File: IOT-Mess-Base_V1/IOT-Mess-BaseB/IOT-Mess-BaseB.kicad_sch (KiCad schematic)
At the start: 23 parts, among them J1 Milk-V Duo, J2 SuperMini_ESP32-H2, J4 Lolin32-Lite, J8 Luat32 C3, SW3 SW_Push, U1 SHT4x, U12 APDS-9960, U13 SHT31-DIS, U17 BH1750FVI-TR, U3 INA219AxDCN

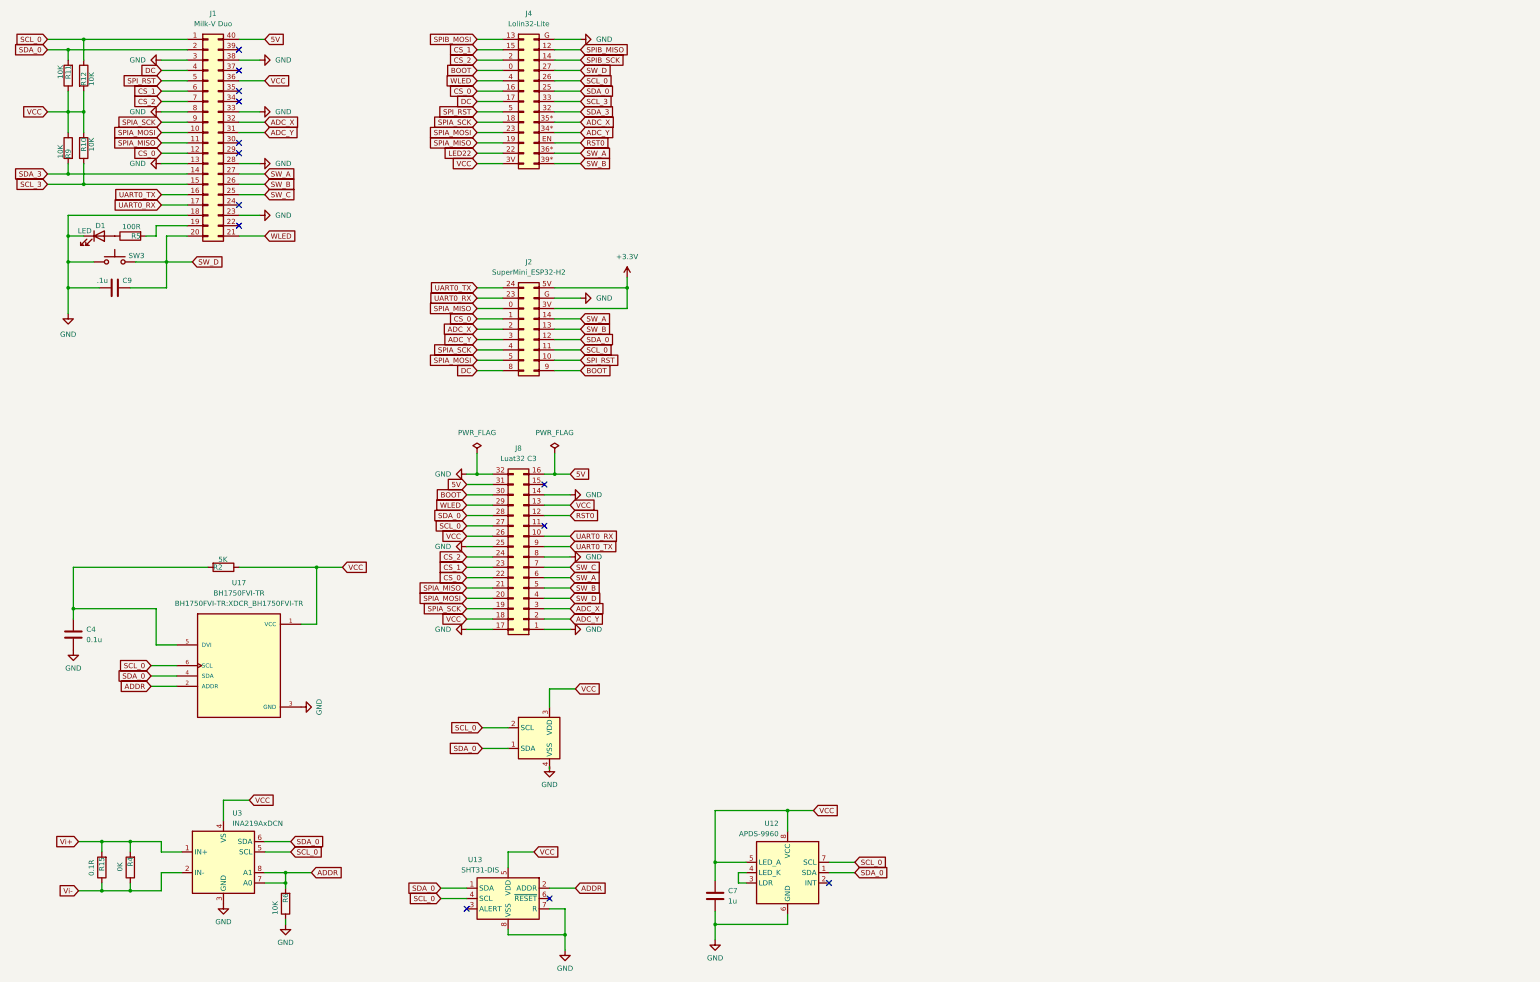
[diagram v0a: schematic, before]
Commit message: did some works.
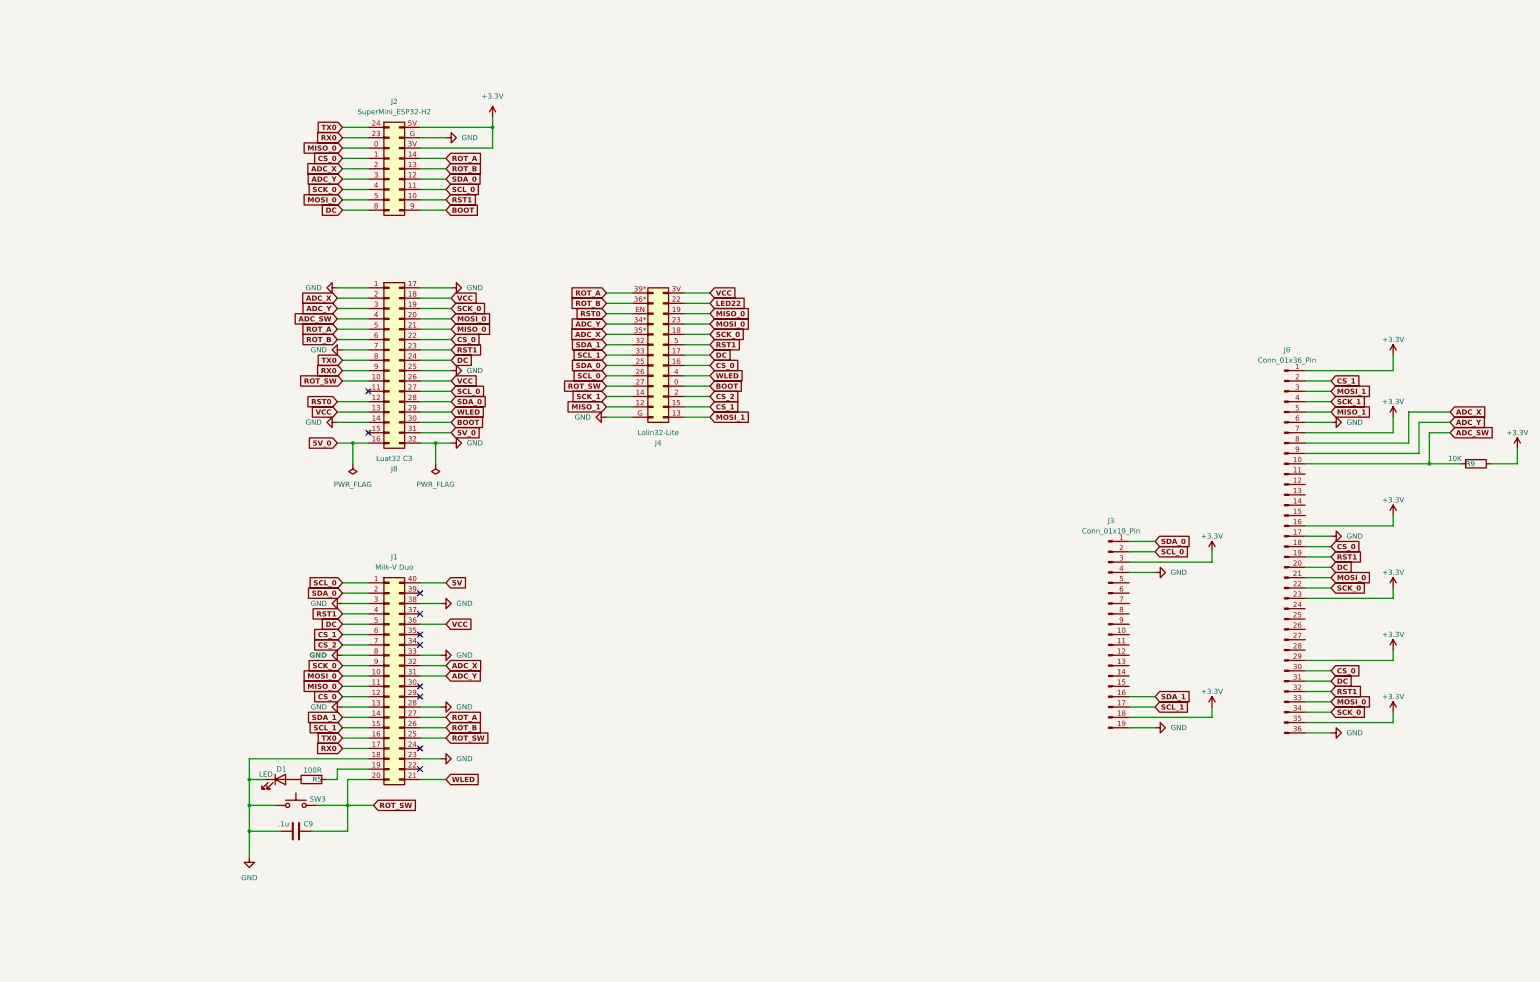
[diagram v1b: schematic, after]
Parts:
- removed C4: 0.1u, Capacitor_SMD:C_0603_1608Metric, symbol Device:C
- removed C7: 1u, Capacitor_SMD:C_0603_1608Metric, symbol Device:C
- removed R10, R11, R12, R6: 10K, Resistor_SMD:R_0603_1608Metric, symbol Device:R
- removed R15: 0.1R, Resistor_SMD:R_2512_6332Metric, symbol Device:R
- removed R2: 5K, Resistor_SMD:R_0603_1608Metric, symbol Device:R
- removed R4: 0K, Jumper:SolderJumper-2_P1.3mm_Open_Pad1.0x1.5mm, symbol Device:R
- removed U1: SHT4x, Sensor_Humidity:Sensirion_DFN-4_1.5x1.5mm_P0.8mm_SHT4x_NoCentralPad, symbol Sensor_Humidity:SHT4x
- removed U12: APDS-9960, Sensor:Avago_APDS-9960, symbol Sensor:APDS-9960
- removed U13: SHT31-DIS, Sensor_Humidity:Sensirion_DFN-8-1EP_2.5x2.5mm_P0.5mm_EP1.1x1.7mm, symbol Sensor_Humidity:SHT31-DIS
- removed U17: BH1750FVI-TR, BH1750FVI-TR:XDCR_BH1750FVI-TR, symbol BH1750FVI-TR:BH1750FVI-TR
- removed U3: INA219AxDCN, Package_TO_SOT_SMD:SOT-23-8, symbol Sensor_Energy:INA219AxDCN
- added J3: Conn_01x19_Pin, Connector_PinHeader_2.54mm:PinHeader_1x19_P2.54mm_Vertical, symbol Connector:Conn_01x19_Pin
- added J6: Conn_01x36_Pin, Connector_PinHeader_2.54mm:PinHeader_1x36_P2.54mm_Vertical, symbol Connector:Conn_01x36_Pin
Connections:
- net +3.3V: now also R9.1, J3.18 (Pin_18), J3.3 (Pin_3), J6.1 (Pin_1), J6.16 (Pin_16), J6.23 (Pin_23), J6.29 (Pin_29), J6.35 (Pin_35), J6.7 (Pin_7)
- net 5V: no longer J8.16 (Pin_16), J8.31 (Pin_31)
- net ADC_X: now also J8.2 (Pin_2), J6.8 (Pin_8); no longer J8.3 (Pin_3)
- net ADC_Y: now also J8.3 (Pin_3), J6.9 (Pin_9); no longer J8.2 (Pin_2)
- net CS_0: now also J6.18 (Pin_18), J6.30 (Pin_30)
- net CS_1: now also J6.2 (Pin_2); no longer J8.23 (Pin_23)
- net CS_2: no longer J8.24 (Pin_24)
- net DC: now also J1.5 (Pin_5), J8.24 (Pin_24), J6.20 (Pin_20), J6.31 (Pin_31); no longer J1.4 (Pin_4)
- net GND: now also J8.7 (Pin_7), J3.19 (Pin_19), J3.4 (Pin_4), J6.17 (Pin_17), J6.36 (Pin_36), J6.6 (Pin_6); no longer J8.8 (Pin_8)
- net SCL_0: now also J3.2 (Pin_2)
- net SDA_0: now also J3.1 (Pin_1)
- net VCC: no longer R9.1
- net SCL_3 renamed SCL_1
- net SCL_1: now also J3.17 (Pin_17)
- net SDA_3 renamed SDA_1
- net SDA_1: now also J3.16 (Pin_16); no longer R9.2
- net SPIA_MISO renamed MISO_0
- net SPIA_MOSI renamed MOSI_0
- net MOSI_0: now also J6.21 (Pin_21), J6.33 (Pin_33)
- net SPIA_SCK renamed SCK_0
- net SCK_0: now also J6.22 (Pin_22), J6.34 (Pin_34)
- net SPIB_MISO renamed MISO_1
- net MISO_1: now also J6.5 (Pin_5)
- net SPIB_MOSI renamed MOSI_1
- net MOSI_1: now also J6.3 (Pin_3)
- net SPIB_SCK renamed SCK_1
- net SCK_1: now also J6.4 (Pin_4)
- net SPI_RST renamed RST1
- net RST1: now also J1.4 (Pin_4), J8.23 (Pin_23), J6.19 (Pin_19), J6.32 (Pin_32); no longer J1.5 (Pin_5)
- net SW_A renamed ROT_A
- net ROT_A: now also J4.39* (Pin_13b), J8.5 (Pin_5); no longer J4.36* (Pin_12b), J8.6 (Pin_6)
- net SW_B renamed ROT_B
- net ROT_B: now also J4.36* (Pin_12b), J8.6 (Pin_6); no longer J4.39* (Pin_13b), J8.5 (Pin_5)
- net SW_C renamed ROT_SW
- net ROT_SW: now also C9.2, J1.20 (Pin_20), J4.27 (Pin_4b), J8.10 (Pin_10), SW3.1; no longer J8.7 (Pin_7)
- removed net SW_D: C9.2, J1.20 (Pin_20), J4.27 (Pin_4b), J8.4 (Pin_4), SW3.1
- net UART0_RX renamed RX0
- net RX0: now also J8.9 (Pin_9); no longer J8.10 (Pin_10)
- net UART0_TX renamed TX0
- net TX0: now also J8.8 (Pin_8); no longer J8.9 (Pin_9)
- new net 5V_0: J8.16 (Pin_16), J8.31 (Pin_31)
- new net ADC_SW: J6.10 (Pin_10), J8.4 (Pin_4), R9.2
- no-connect marks 13 -> 10
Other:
- moved on the sheet: C9, D1, J1, J2, J4, J8, R5, SW3

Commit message: did some works.
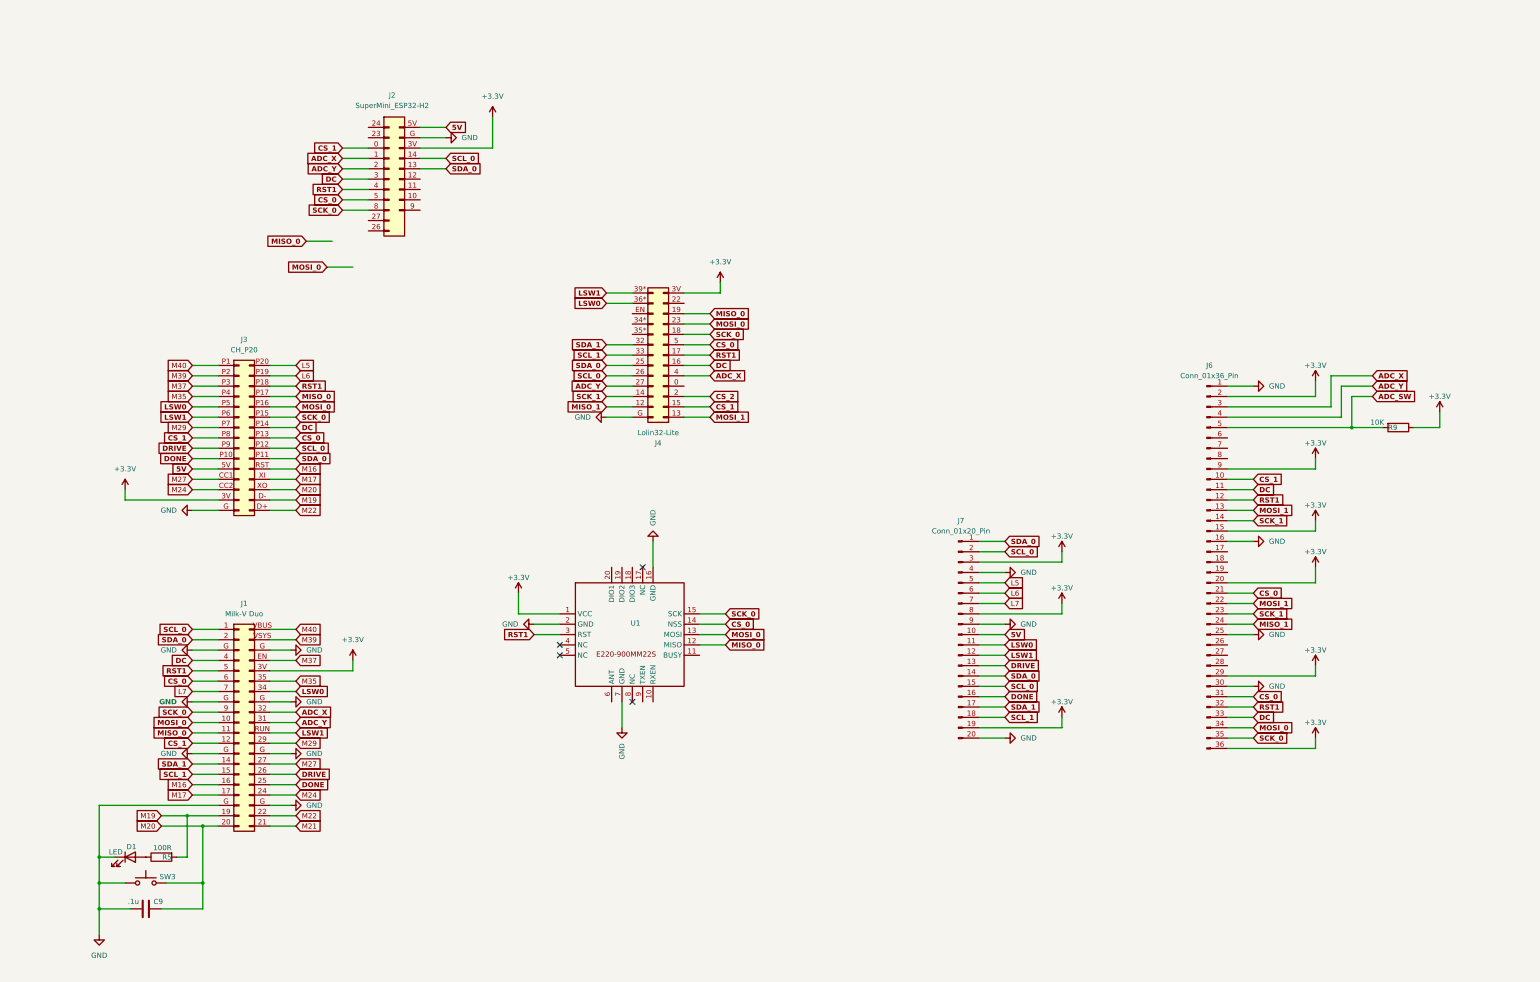
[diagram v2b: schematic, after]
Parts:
- removed J3: Conn_01x19_Pin, Connector_PinHeader_2.54mm:PinHeader_1x19_P2.54mm_Vertical, symbol Connector:Conn_01x19_Pin
- removed J8: Luat32 C3, IOT-Mess-Footprints:Luat32 C3, symbol Connector_Generic:Conn_02x16_Top_Bottom
- added J3: CH_P20, IOT-Mess-Footprints:CH_P20, symbol IOT-Mess:CH_P20
- added J7: Conn_01x20_Pin, Connector_PinHeader_2.54mm:PinHeader_1x20_P2.54mm_Vertical, symbol Connector:Conn_01x20_Pin
- added U1: ~, IOT-Mess-Footprints:E220-900, symbol IOT-Mess:E220-900
- J2: footprint (none) -> IOT-Mess-Footprints:SuperMiniH2
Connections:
- net +3.3V: now also J1.3V (Pin_36), J4.3V (Pin_13a), J6.15 (Pin_15), J6.2 (Pin_2), J6.20 (Pin_20), J6.36 (Pin_36), J6.9 (Pin_9), J3.3V (Pin_14), J7.19 (Pin_19), J7.3 (Pin_3), J7.8 (Pin_8), U1.1 (VCC); no longer J2.5V (Pin_18), J6.1 (Pin_1), J6.16 (Pin_16), J6.23 (Pin_23), J6.35 (Pin_35), J6.7 (Pin_7)
- net 5V: now also J2.5V (Pin_18), J3.5V (Pin_11), J7.10 (Pin_10); no longer J1.40 (Pin_40)
- net ADC_SW: now also J6.5 (Pin_5); no longer J6.10 (Pin_10)
- net ADC_X: now also J2.1 (Pin_4), J4.4 (Pin_5a), J6.3 (Pin_3); no longer J2.2 (Pin_5), J4.35* (Pin_9b), J6.8 (Pin_8)
- net ADC_Y: now also J2.2 (Pin_5), J4.27 (Pin_4b), J6.4 (Pin_4); no longer J2.3 (Pin_6), J4.34* (Pin_10b), J6.9 (Pin_9)
- net CS_0: now also J1.6 (Pin_6), J2.5 (Pin_8), J4.5 (Pin_8a), J6.21 (Pin_21), J6.31 (Pin_31), J3.P13 (Pin_23), U1.14 (NSS); no longer J1.12 (Pin_12), J2.1 (Pin_4), J4.16 (Pin_6a), J6.18 (Pin_18), J6.30 (Pin_30)
- net CS_1: now also J1.12 (Pin_12), J2.0 (Pin_3), J6.10 (Pin_10), J3.P8 (Pin_8); no longer J1.6 (Pin_6), J6.2 (Pin_2)
- net CS_2: no longer J1.7 (Pin_7)
- net DC: now also J1.4 (Pin_4), J2.3 (Pin_6), J4.16 (Pin_6a), J6.11 (Pin_11), J6.33 (Pin_33), J3.P14 (Pin_22); no longer J1.5 (Pin_5), J2.8 (Pin_9), J4.17 (Pin_7a), J6.20 (Pin_20), J6.31 (Pin_31)
- net GND: now also J1.G (Pin_23), J6.1 (Pin_1), J6.16 (Pin_16), J6.25 (Pin_25), J6.30 (Pin_30), J3.G (Pin_15), J7.20 (Pin_20), J7.4 (Pin_4), J7.9 (Pin_9), U1.16 (GND), U1.2 (GND), U1.7 (GND); no longer J1.13 (Pin_13), J1.18 (Pin_18), J1.23 (Pin_23), J1.28 (Pin_28), J1.3 (Pin_3), J1.33 (Pin_33), J1.38 (Pin_38), J1.8 (Pin_8), J6.17 (Pin_17), J6.36 (Pin_36), J6.6 (Pin_6)
- net MISO_0: now also J3.P17 (Pin_19), U1.12 (MISO); no longer J2.0 (Pin_3)
- net MISO_1: now also J6.24 (Pin_24); no longer J6.5 (Pin_5)
- net MOSI_0: now also J6.34 (Pin_34), J3.P16 (Pin_20), U1.13 (MOSI); no longer J2.5 (Pin_8), J6.21 (Pin_21), J6.33 (Pin_33)
- net MOSI_1: now also J6.13 (Pin_13), J6.22 (Pin_22); no longer J6.3 (Pin_3)
- net RST1: now also J1.5 (Pin_5), J2.4 (Pin_7), J4.17 (Pin_7a), J6.12 (Pin_12), J3.P18 (Pin_18), U1.3 (RST); no longer J1.4 (Pin_4), J2.10 (Pin_11), J4.5 (Pin_8a), J6.19 (Pin_19)
- net SCK_0: now also J2.8 (Pin_9), J6.35 (Pin_35), J3.P15 (Pin_21), U1.15 (SCK); no longer J2.4 (Pin_7), J6.22 (Pin_22), J6.34 (Pin_34)
- net SCK_1: now also J6.14 (Pin_14), J6.23 (Pin_23); no longer J6.4 (Pin_4)
- net SCL_0: now also J2.14 (Pin_15), J3.P12 (Pin_24), J7.15 (Pin_15), J7.2 (Pin_2); no longer J2.11 (Pin_12)
- net SCL_1: now also J7.18 (Pin_18)
- net SDA_0: now also J2.13 (Pin_14), J3.P11 (Pin_25), J7.1 (Pin_1), J7.14 (Pin_14); no longer J2.12 (Pin_13)
- net SDA_1: now also J7.17 (Pin_17)
- net M19: now reaches J1.19 (Pin_19), R5.2
- net M19: now also J3.D- (Pin_29)
- net M22: now reaches J1.22 (Pin_22)
- net M22: now also J3.D+ (Pin_30)
- net M24: now reaches J1.24 (Pin_24)
- net M24: now also J3.CC2 (Pin_13)
- net M29: now reaches J1.29 (Pin_29)
- net M29: now also J3.P7 (Pin_7)
- net LSW0: now reaches J1.34 (Pin_34)
- net LSW0: now also J4.36* (Pin_12b), J3.P5 (Pin_5), J7.11 (Pin_11)
- net M35: now reaches J1.35 (Pin_35)
- net M35: now also J3.P4 (Pin_4)
- net BOOT: no longer names the net of J4.0 (Pin_4a)
- net BOOT: no longer J2.9 (Pin_10)
- net LED22: no longer names the net of J4.22 (Pin_12a)
- removed net ROT_A: J1.27 (Pin_27), J2.14 (Pin_15), J4.39* (Pin_13b)
- removed net ROT_B: J1.26 (Pin_26), J2.13 (Pin_14), J4.36* (Pin_12b)
- net ROT_SW renamed M20
- net M20: now also J3.XO (Pin_28); no longer J1.25 (Pin_25), J4.27 (Pin_4b)
- net RST0: no longer names the net of J4.EN (Pin_11b)
- net RX0: no longer names the net of J2.23 (Pin_2)
- net RX0: no longer J1.17 (Pin_17)
- net TX0: no longer names the net of J2.24 (Pin_1)
- net TX0: no longer J1.16 (Pin_16)
- removed net VCC: J1.36 (Pin_36), J4.3V (Pin_13a)
- net WLED renamed M21
- net M21: no longer J4.4 (Pin_5a)
- new net DONE: J1.25 (Pin_25), J3.P10 (Pin_10), J7.16 (Pin_16)
- new net DRIVE: J1.26 (Pin_26), J3.P9 (Pin_9), J7.13 (Pin_13)
- new net L5: J3.P20 (Pin_16), J7.5 (Pin_5)
- new net L6: J3.P19 (Pin_17), J7.6 (Pin_6)
- new net L7: J1.7 (Pin_7), J7.7 (Pin_7)
- new net LSW1: J1.RUN (Pin_30), J3.P6 (Pin_6), J4.39* (Pin_13b), J7.12 (Pin_12)
- new net M16: J1.16 (Pin_16), J3.RST (Pin_26)
- new net M17: J1.17 (Pin_17), J3.XI (Pin_27)
- new net M27: J1.27 (Pin_27), J3.CC1 (Pin_12)
- new net M37: J1.EN (Pin_37), J3.P3 (Pin_3)
- new net M39: J1.VSYS (Pin_39), J3.P2 (Pin_2)
- new net M40: J1.VBUS (Pin_40), J3.P1 (Pin_1)
- no-connect marks 10 -> 4
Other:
- moved on the sheet: C9, D1, J1, J6, R5, R9, SW3
